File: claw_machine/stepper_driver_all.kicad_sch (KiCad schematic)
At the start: 0 parts

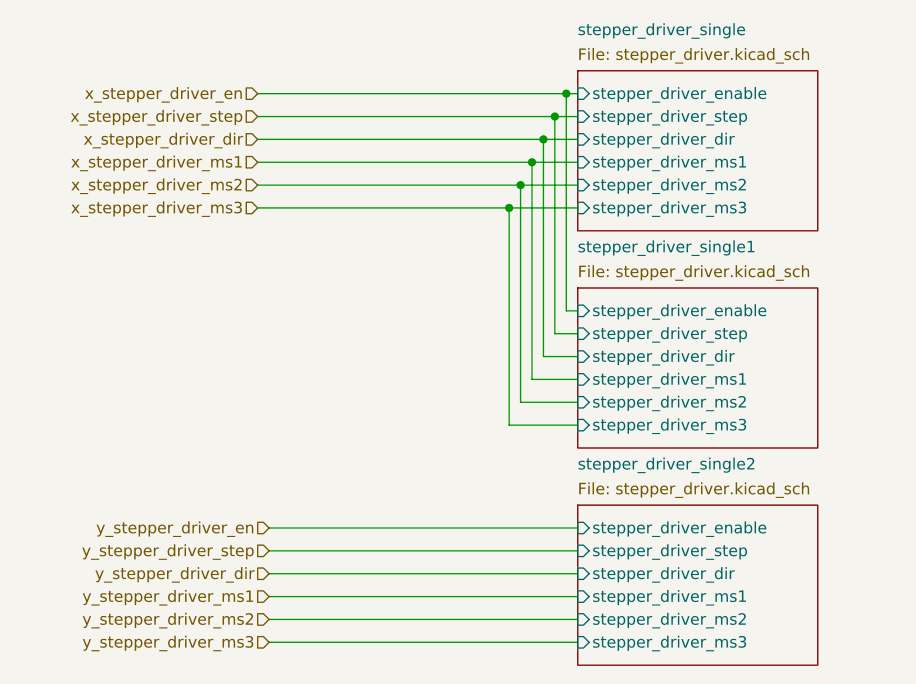
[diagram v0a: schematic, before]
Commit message: Rework schematic
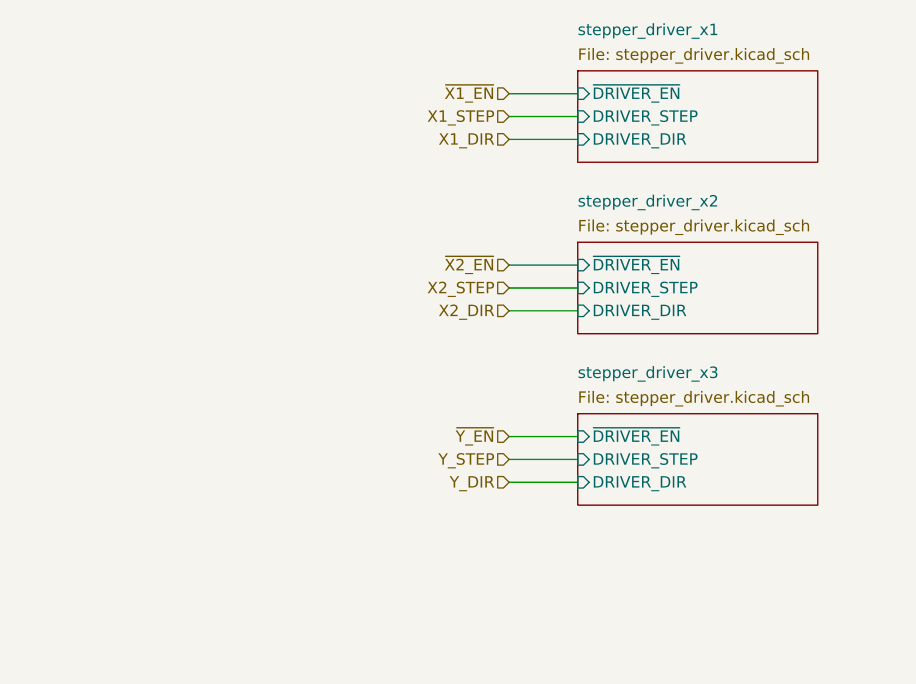
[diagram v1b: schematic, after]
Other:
- sheet stepper_driver_single renamed stepper_driver_x1
- removed sheet stepper_driver_single1
- removed sheet stepper_driver_single2
- added sheet stepper_driver_x2 (stepper_driver.kicad_sch)
- added sheet stepper_driver_x3 (stepper_driver.kicad_sch)
- sheet stepper_driver_x1 ports: added DRIVER_DIR, DRIVER_STEP, ~{DRIVER_EN}; removed stepper_driver_dir, stepper_driver_enable, stepper_driver_ms1, stepper_driver_ms2, stepper_driver_ms3, stepper_driver_step
